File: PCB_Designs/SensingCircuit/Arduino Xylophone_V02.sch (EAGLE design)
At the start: 92 parts, among them IC1 MCP601OT, IC10 MCP601OT, IC11 MCP601OT, IC12 MCP601OT, IC13 MCP601OT, IC2 MCP601OT, IC3 MCP601OT, IC4 MCP601OT, IC5 MCP601OT, IC6 MCP601OT, IC7 MCP601OT, IC8 MCP601OT, IC9 MCP601OT, U1 ATMEGA2560AU

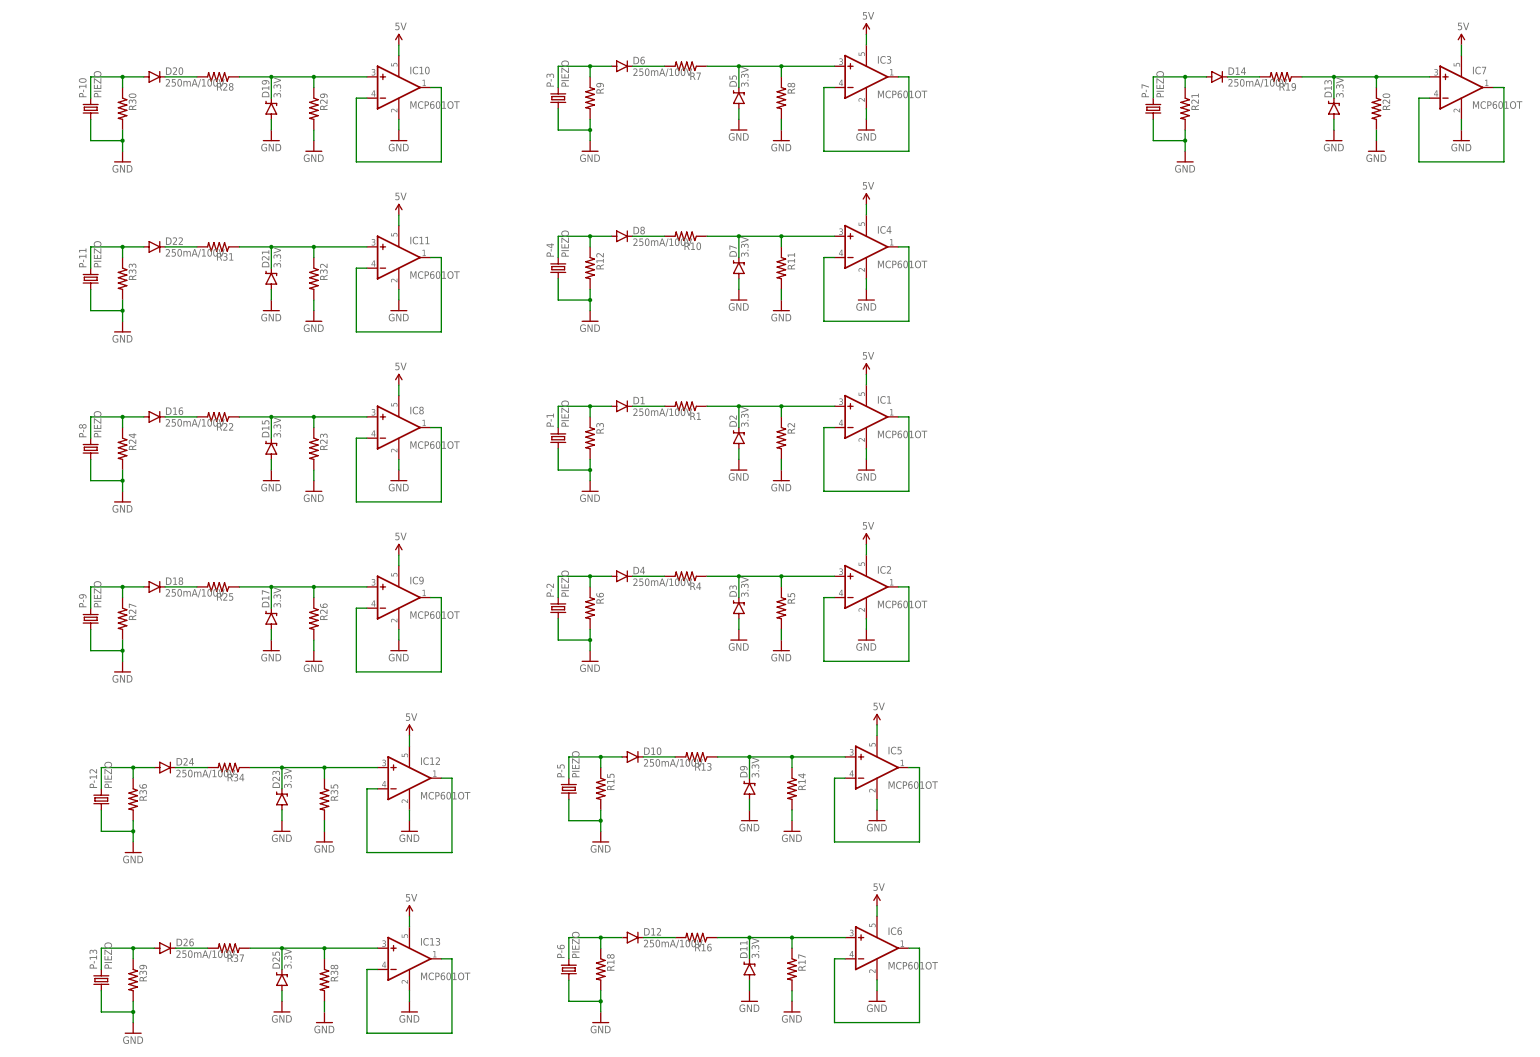
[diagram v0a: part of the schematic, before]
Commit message: working on board layout for Xylophone sensing circuit
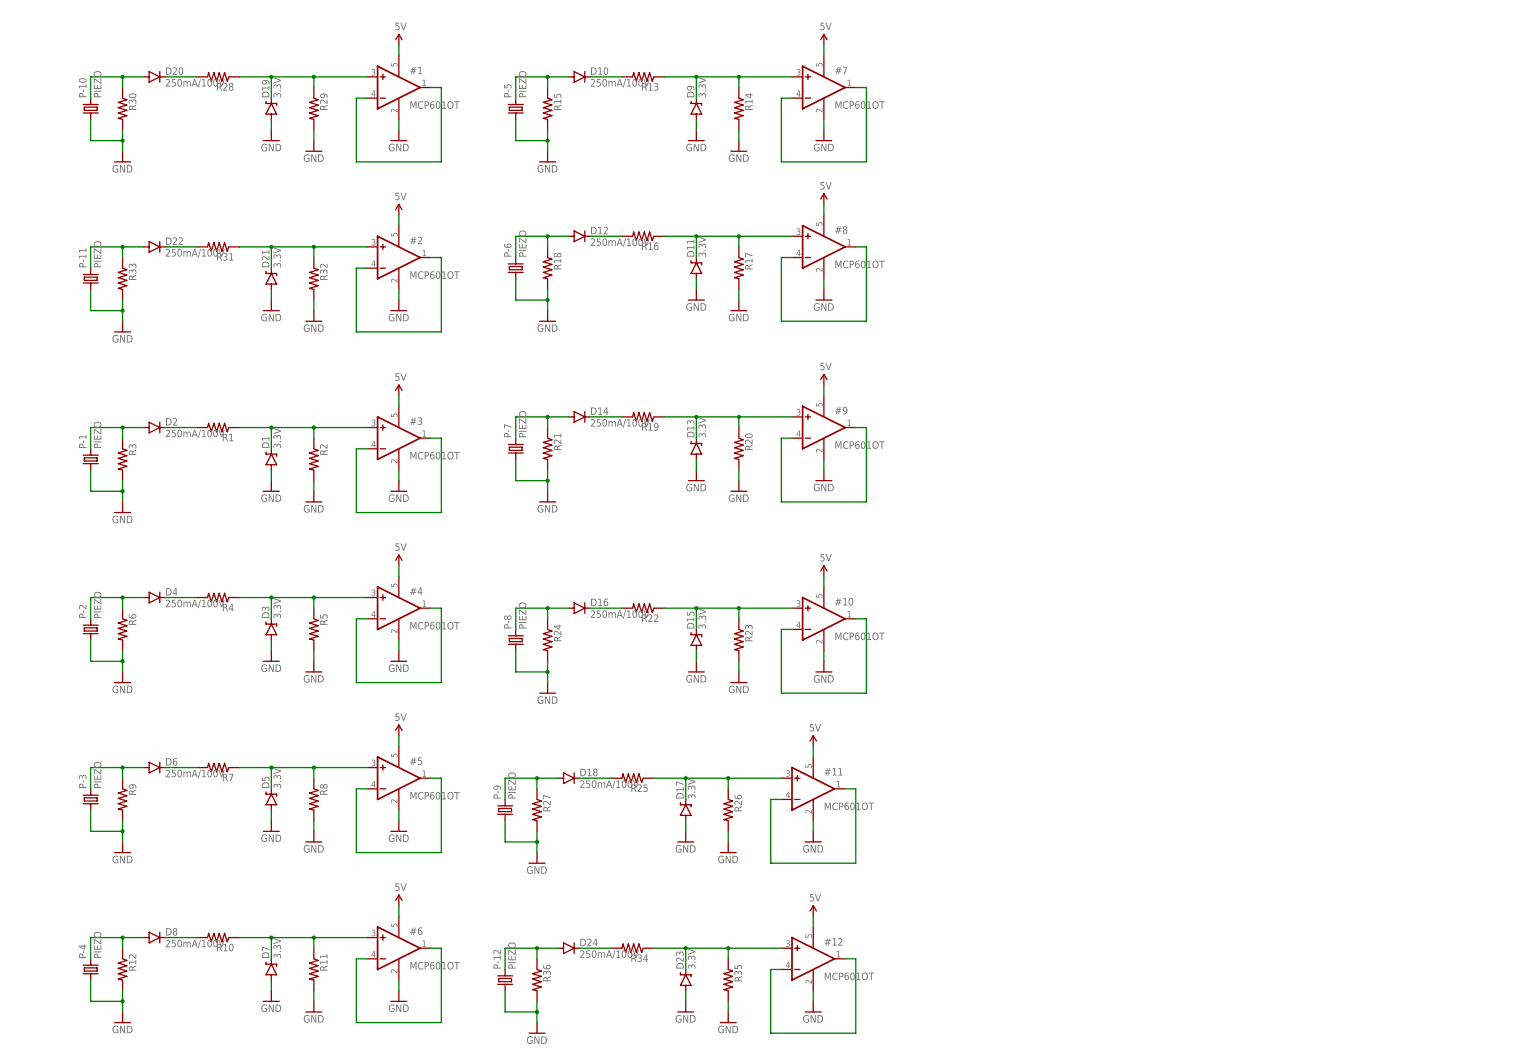
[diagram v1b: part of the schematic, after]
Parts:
- removed D25: 3.3V, SparkFun-DiscreteSemi:DIODE-ZENER3.3V
- removed D26: 250mA/100V, SparkFun-DiscreteSemi:DIODEBAS16
- removed IC1, IC12, IC13, IC2, IC3, IC4, IC5, IC6, IC7, IC8, IC9: MCP601OT, linear:MCP601OT
- removed P-13: PIEZO, Orlando:PIEZO-LEADED
- removed R37, R38, R39: (no value), resistor:R-US_R0402
- added #10, #11, #12, #3, #4, #5, #6, #7, #8, #9: MCP601OT, linear:MCP601OT
- D1: value 250mA/100V -> 3.3V; device SparkFun-DiscreteSemi:DIODEBAS16 -> SparkFun-DiscreteSemi:DIODE-ZENER3.3V
- D2: value 3.3V -> 250mA/100V; device SparkFun-DiscreteSemi:DIODE-ZENER3.3V -> SparkFun-DiscreteSemi:DIODEBAS16
- renumbered IC10 to #1, IC11 to #2
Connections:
- removed net N$49: D25.C, IC13.+IN, R37.1, R38.1
- removed net N$50: D26.C, R37.2
- removed net N$51: IC13.-IN, IC13.OUT
- removed net N$52: D26.A, P-13.2, R39.1
- net 5V: now also #10.V+, #11.V+, #12.V+, #3.V+, #4.V+, #5.V+, #6.V+, #7.V+, #8.V+, #9.V+; no longer IC1.V+, IC12.V+, IC13.V+, IC2.V+, IC3.V+, IC4.V+, IC5.V+, IC6.V+, IC7.V+, IC8.V+, IC9.V+
- net GND: now also #10.V-, #11.V-, #12.V-, #3.V-, #4.V-, #5.V-, #6.V-, #7.V-, #8.V-, #9.V-, D1.A; no longer D2.A, D25.A, IC1.V-, IC12.V-, IC13.V-, IC2.V-, IC3.V-, IC4.V-, IC5.V-, IC6.V-, IC7.V-, IC8.V-, IC9.V-, P-13.1, R38.2, R39.2
- net N$1: now also #3.+IN, D1.C; no longer D2.C, IC1.+IN
- net N$11: now also #5.-IN, #5.OUT; no longer IC3.-IN, IC3.OUT
- net N$13: now also #6.+IN; no longer IC4.+IN
- net N$15: now also #6.-IN, #6.OUT; no longer IC4.-IN, IC4.OUT
- net N$17: now also #7.+IN; no longer IC5.+IN
- net N$19: now also #7.-IN, #7.OUT; no longer IC5.-IN, IC5.OUT
- net N$2: now also D2.C; no longer D1.C
- net N$21: now also #8.+IN; no longer IC6.+IN
- net N$23: now also #8.-IN, #8.OUT; no longer IC6.-IN, IC6.OUT
- net N$25: now also #9.+IN; no longer IC7.+IN
- net N$27: now also #9.-IN, #9.OUT; no longer IC7.-IN, IC7.OUT
- net N$29: now also #10.+IN; no longer IC8.+IN
- net N$3: now also #3.-IN, #3.OUT; no longer IC1.-IN, IC1.OUT
- net N$31: now also #10.-IN, #10.OUT; no longer IC8.-IN, IC8.OUT
- net N$33: now also #11.+IN; no longer IC9.+IN
- net N$35: now also #11.-IN, #11.OUT; no longer IC9.-IN, IC9.OUT
- net N$4: now also D2.A; no longer D1.A
- net N$45: now also #12.+IN; no longer IC12.+IN
- net N$47: now also #12.-IN, #12.OUT; no longer IC12.-IN, IC12.OUT
- net N$5: now also #4.+IN; no longer IC2.+IN
- net N$7: now also #4.-IN, #4.OUT; no longer IC2.-IN, IC2.OUT
- net N$9: now also #5.+IN; no longer IC3.+IN
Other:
- moved on the sheet: D10, D11, D12, D13, D14, D15, D16, D17, D18, D23, D24, D3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
